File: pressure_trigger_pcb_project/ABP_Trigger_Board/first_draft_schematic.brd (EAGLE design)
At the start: 67 x 39.4 mm, 28 parts, among them U1 OPA4340UA

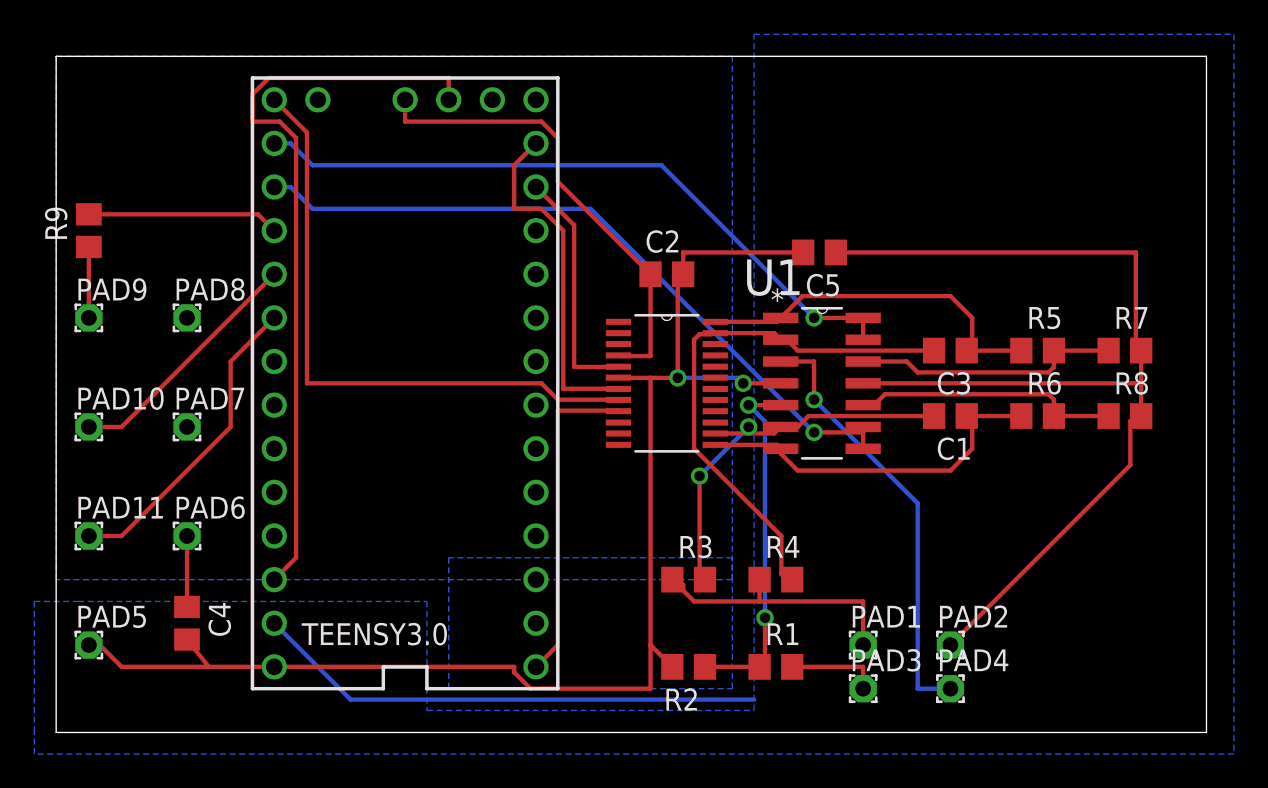
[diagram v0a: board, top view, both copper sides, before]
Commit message: new board layout
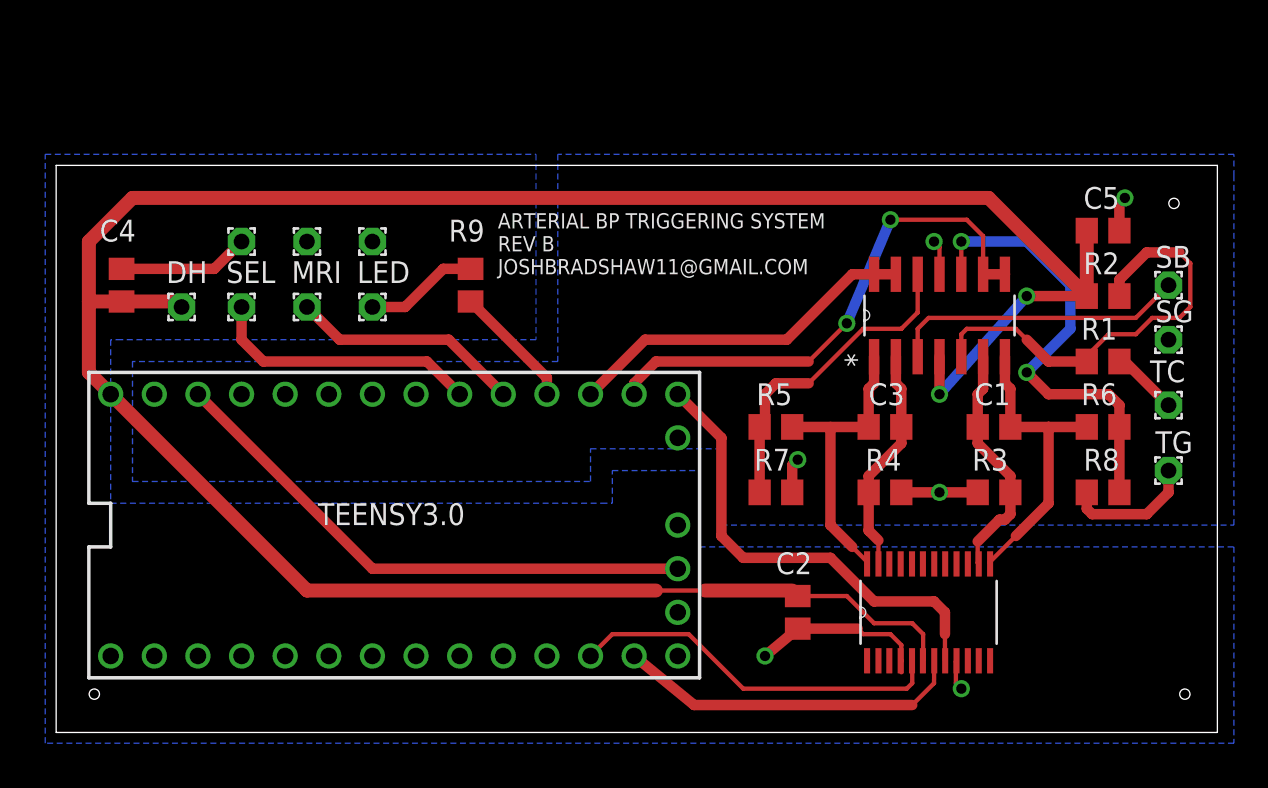
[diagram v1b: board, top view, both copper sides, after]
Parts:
- removed AD5206: AD5206BRUZ10, AD5206:SOP65P640X120-24N
- removed PAD1, PAD10, PAD11, PAD2, PAD3, PAD5, PAD9: WIREPAD1,6/0,9, wirepad:1,6/0,9
- removed PAD4: SAMBA, wirepad:1,6/0,9
- added AD5206-50: AD5206BRUZ10, AD5206:SOP65P640X120-24N
- added DH, LED, MRI, SEL, SG, TC, TG: WIREPAD1,6/0,9, wirepad:1,6/0,9
- added SB: SAMBA, wirepad:1,6/0,9
- moved R2 32.4 mm to (61.0, 25.4)
- moved R1 26.1 mm to (61.0, 21.6)
- moved R9 22.5 mm to (24.1, 26.0), turned to 270 degrees
- moved R7 21.9 mm to (41.9, 14.0)
- moved C2 21.1 mm to (43.2, 6.99), turned to 90 degrees
- moved C4 20.1 mm to (3.81, 26.0)
- moved R3 18.5 mm to (54.6, 14.0)
- moved PAD6 17.4 mm to (10.8, 28.6), turned to 270 degrees
- moved C5 16.6 mm to (61.0, 29.2)
- moved R5 15.9 mm to (41.9, 17.8), turned to 180 degrees
- moved U1 13.1 mm to (55.2, 26.7), turned to 90 degrees
- moved PAD7 12.9 mm to (14.6, 28.6), turned to 270 degrees
- moved PAD8 11.7 mm to (18.4, 28.6), turned to 270 degrees
- moved TEENSY3.0 8.28 mm to (19.7, 12.1), turned to 90 degrees
- moved R4 8.13 mm to (48.3, 14.0), turned to 180 degrees
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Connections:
- net AGND: now also SG.1, TG.1; no longer PAD1.1, PAD2.1
- net GND: now also AD5206-50.4, AD5206-50.9; no longer AD5206.4, AD5206.9
- net N$1: now also TEENSY3.0.15/A1; no longer TEENSY3.0.14/A0
- net N$10: now also SB.1; no longer PAD4.1
- net N$11: now also LED.1; no longer PAD9.1
- net N$12: now also AD5206-50.14; no longer AD5206.14
- net N$13: now also TC.1; no longer PAD3.1
- net N$15: now also MRI.1; no longer PAD10.1
- net N$16: now also SEL.1; no longer PAD11.1
- net N$17: now also AD5206-50.13; no longer AD5206.13
- net N$19: now also AD5206-50.8; no longer AD5206.8
- net N$2: now also TEENSY3.0.14/A0; no longer TEENSY3.0.15/A1
- net N$3: now also AD5206-50.23; no longer AD5206.23
- net N$5: now also AD5206-50.24; no longer AD5206.24
- net N$7: now also AD5206-50.5; no longer AD5206.5
- net N$8: now also AD5206-50.7; no longer AD5206.7
- net VCC: now also AD5206-50.6, DH.1; no longer AD5206.6, PAD5.1
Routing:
- net AGND: track 107.0 -> 18.2 mm, vias 0 -> 4
- net VCC: track 80.1 -> 149.3 mm
- net GND: track 50.5 -> 19.9 mm, vias 0 -> 2
- net N$1: track 39.8 -> 20.7 mm, vias 1 -> 0
- net N$3: track 31.1 -> 13.2 mm
- net 3.3V: track 43.9 -> 32.1 mm
- net N$2: track 41.5 -> 30.3 mm, vias 1 -> 2
- net N$9: track 15.6 -> 26.7 mm, vias 0 -> 2
- net N$12: track 23.9 -> 14.0 mm, vias 2 -> 0
- net N$19: track 35.8 -> 27.0 mm
- net N$10: track 25.4 -> 17.3 mm, vias 1 -> 0
- net N$7: track 14.0 -> 22.0 mm
- net N$4: track 21.0 -> 25.6 mm, vias 2 -> 0
- net N$14: track 11.2 -> 7.24 mm
- net N$5: track 21.3 -> 17.5 mm
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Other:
- board size 67 x 39.4 mm -> 67.6 x 33 mm
- board text added: "ARTERIAL BP TRIGGERING SYSTEM REV B JOSHBRADSHAW11@GMAIL.COM"
